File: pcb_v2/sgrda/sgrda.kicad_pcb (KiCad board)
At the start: 2 copper layers, 43.5 x 61 mm, 17 parts, among them J1 addr_decoder, U1 74HC238, U2 74LS138, U4 74LS04

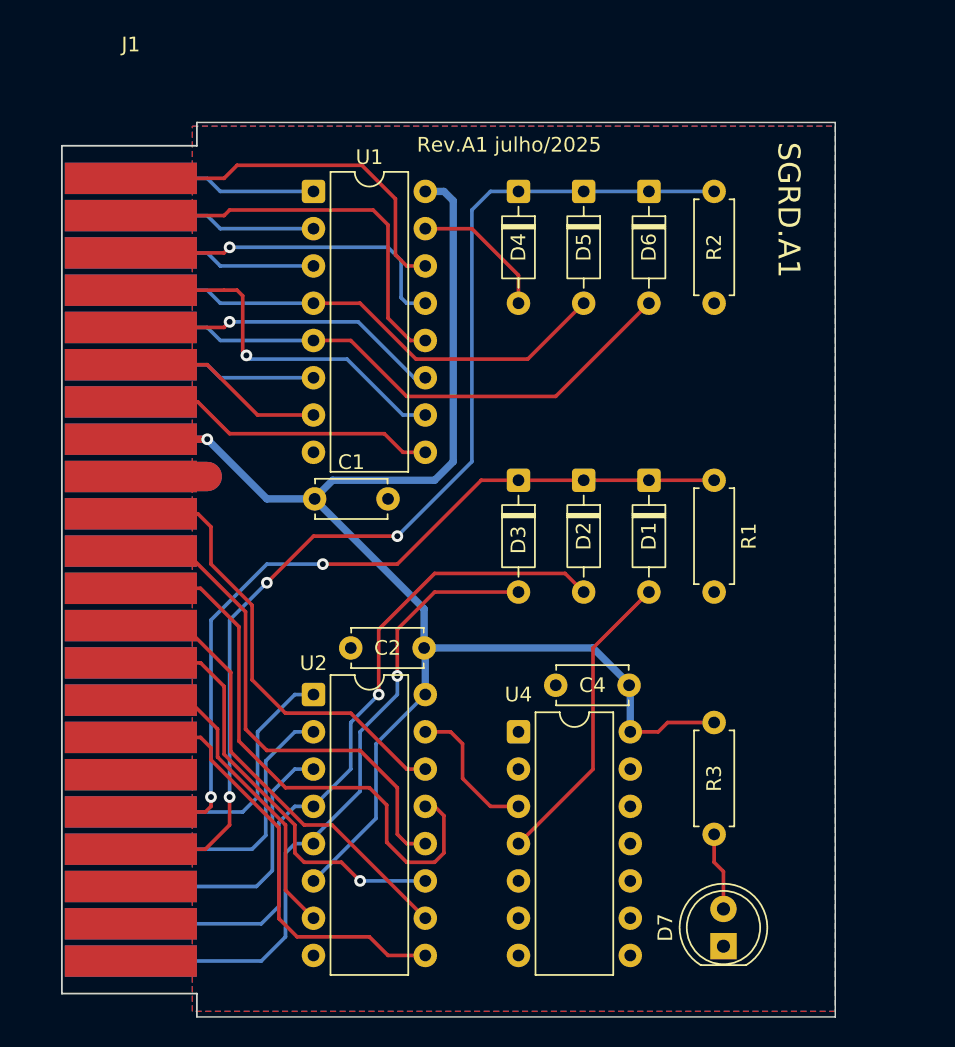
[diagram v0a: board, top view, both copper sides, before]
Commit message: arquivos do gdrive
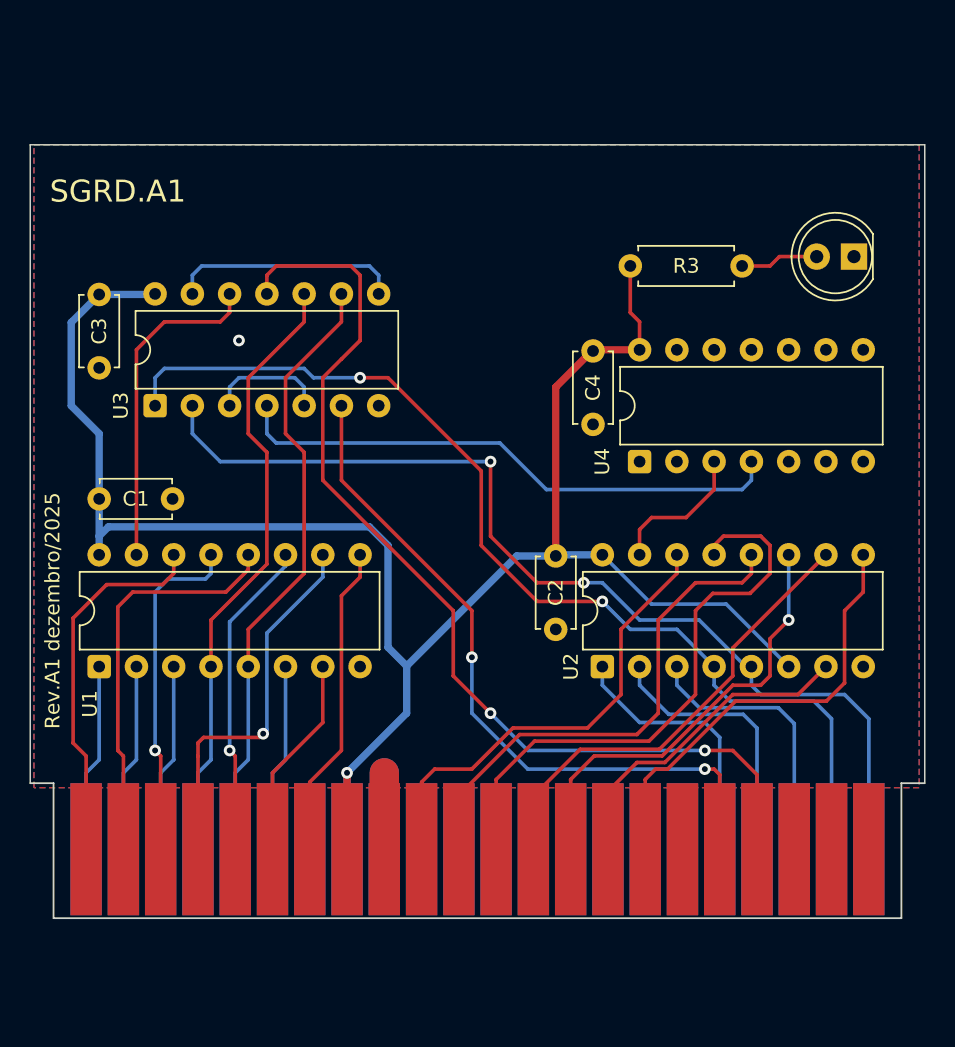
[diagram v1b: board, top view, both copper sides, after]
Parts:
- removed D1, D2, D3, D4, D5, D6: 1N4148, Diode_THT:D_DO-35_SOD27_P7.62mm_Horizontal
- removed R1, R2: 4.7K, Resistor_THT:R_Axial_DIN0207_L6.3mm_D2.5mm_P7.62mm_Horizontal
- added C3: 100nF, Capacitor_THT:C_Disc_D4.7mm_W2.5mm_P5.00mm, F.Cu at (55.2, 41.3)
- added U3: 74LS32, Package_DIP:DIP-14_W7.62mm, F.Cu at (59.1, 48.9)
- D7: value LED -> POWER
- moved D7 47.8 mm to (106.7, 38.7), turned to 180 degrees
- moved J1 45.8 mm to (54.4, 79.1), turned to 90 degrees
- moved R3 38.8 mm to (99.1, 39.4), turned to 180 degrees
- moved U1 35.5 mm to (55.2, 66.7), turned to 90 degrees
- moved C4 22.9 mm to (88.9, 45.2), turned to -90 degrees
- moved U4 20.2 mm to (92.1, 52.7), turned to 90 degrees
- moved U2 19.8 mm to (89.5, 66.7), turned to 90 degrees
- moved C1 14.7 mm to (55.2, 55.2)
- moved C2 10.9 mm to (86.4, 59.1), turned to -90 degrees
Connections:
- net n_read_A renamed ~{read_A}
- net n_read_B renamed ~{read_B}
- net n_read_C renamed ~{read_C}
- net n_read_D renamed ~{read_D}
- net n_read_E renamed ~{read_E}
- net n_read_H renamed ~{read_H}
- net n_read_L renamed ~{read_L}
- U4 pad 1: unconnected-(U4-Pad1) -> GND
- U4 pad 11: unconnected-(U4-Pad11) -> GND
- U4 pad 13: unconnected-(U4-Pad13) -> GND
- U4 pad 5: unconnected-(U4-Pad5) -> GND
- U4 pad 9: unconnected-(U4-Pad9) -> GND
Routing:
- net rd_addr_4: track 45.4 -> 68.7 mm, vias 1 -> 2
- net +5V: track 106.7 -> 128.5 mm
- net rd_addr_3: track 49.1 -> 70.8 mm, vias 1 -> 2
- net read_zero: track 20.8 -> 38.0 mm
- net Net-(U3-Pad13): track 0.00 -> 15.8 mm
- net write_zero: track 9.57 -> 22.6 mm
- net Net-(U3-Pad3): track 0.00 -> 8.78 mm
- net ~{enable_data_out}: track 56.6 -> 48.3 mm
- net ~{enable_data_in}: track 76.5 -> 68.8 mm, vias 3 -> 2
- net wr_addr_3: track 34.4 -> 41.9 mm
- net wr_addr_4: track 39.9 -> 41.9 mm
- net GND: vias 0 -> 1
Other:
- board size 43.5 x 61 mm -> 61 x 43.5 mm
- board text added: "Rev.A1 dezembro/2025"
- board text removed: "Rev.A1 julho/2025"
